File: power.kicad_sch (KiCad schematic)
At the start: 28 parts, among them J2 USB_C_Receptacle_USB2.0, U4 XC6220B331MR, U5 TLV70237_SOT23-5, U6 SRV05-4

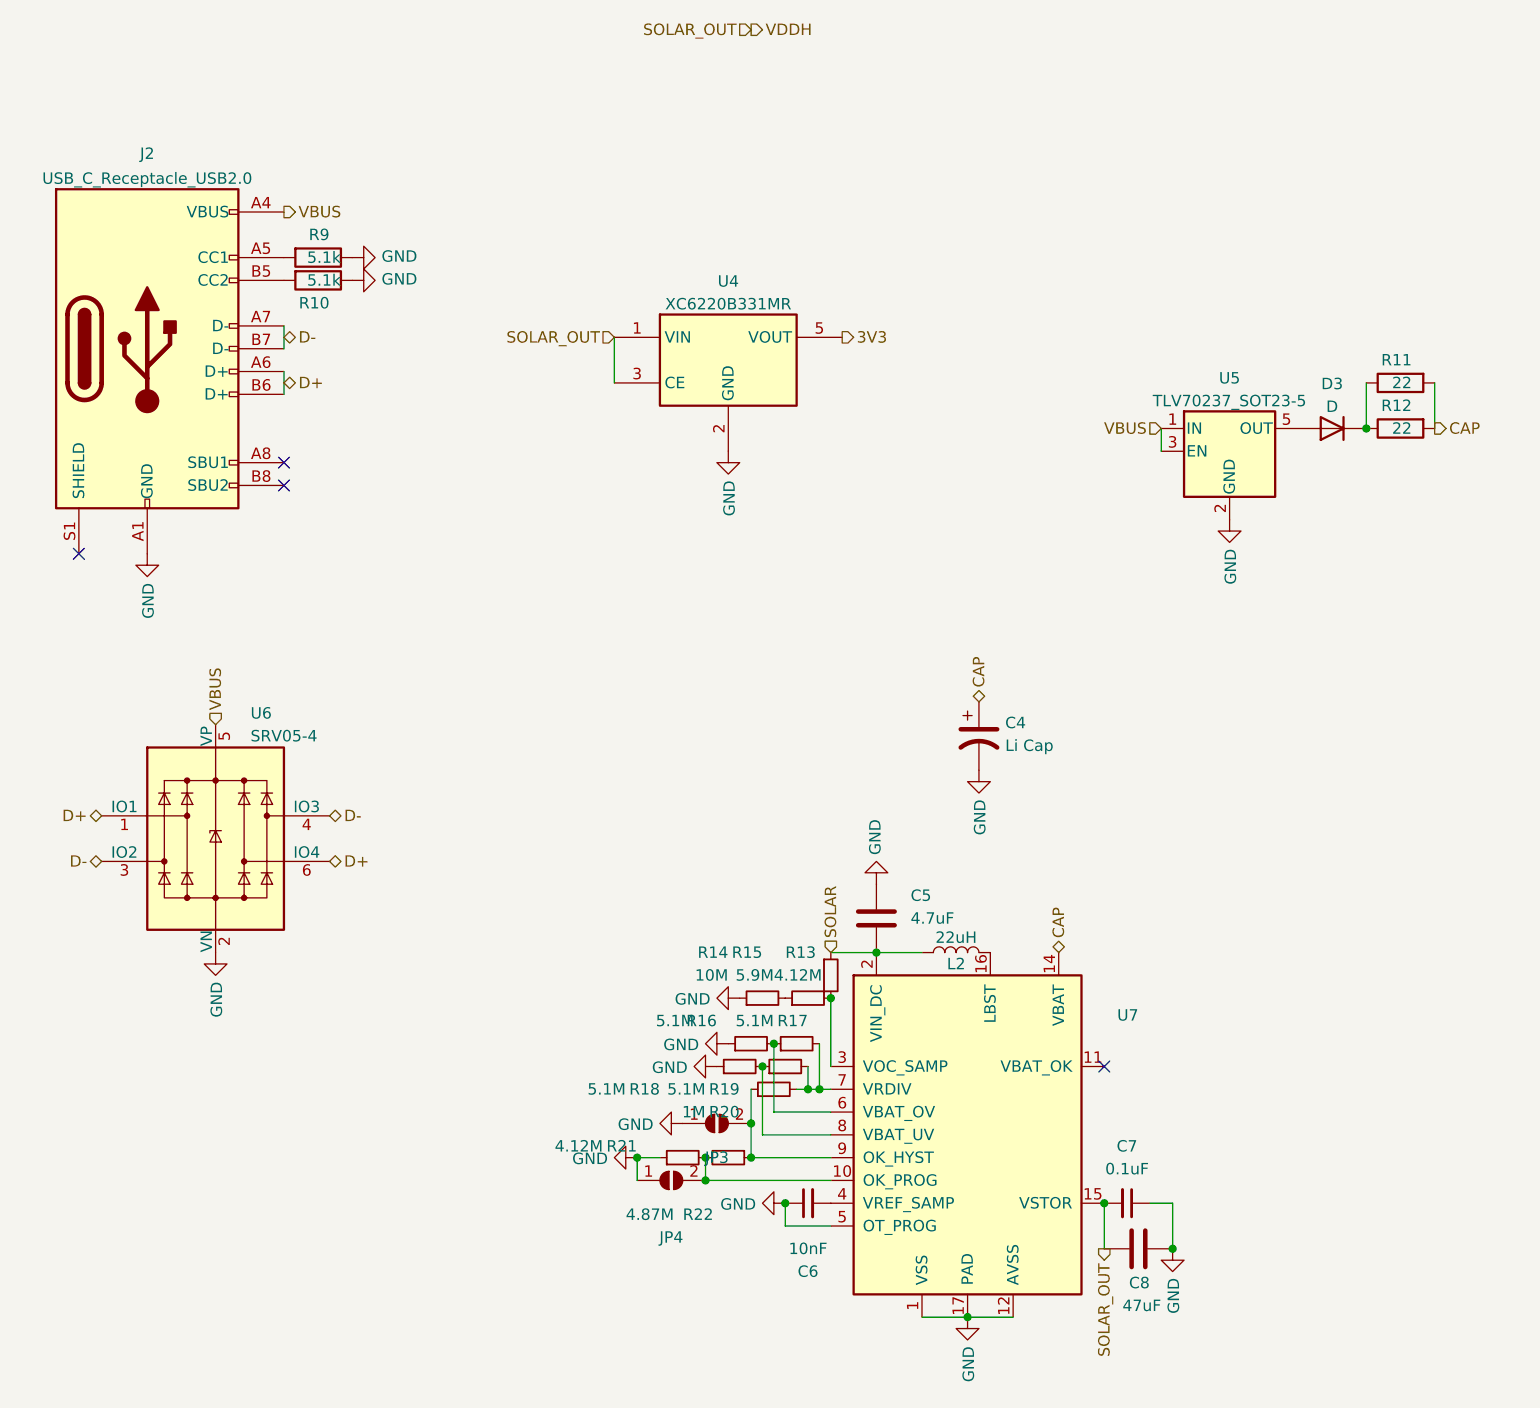
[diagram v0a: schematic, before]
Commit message: no screen
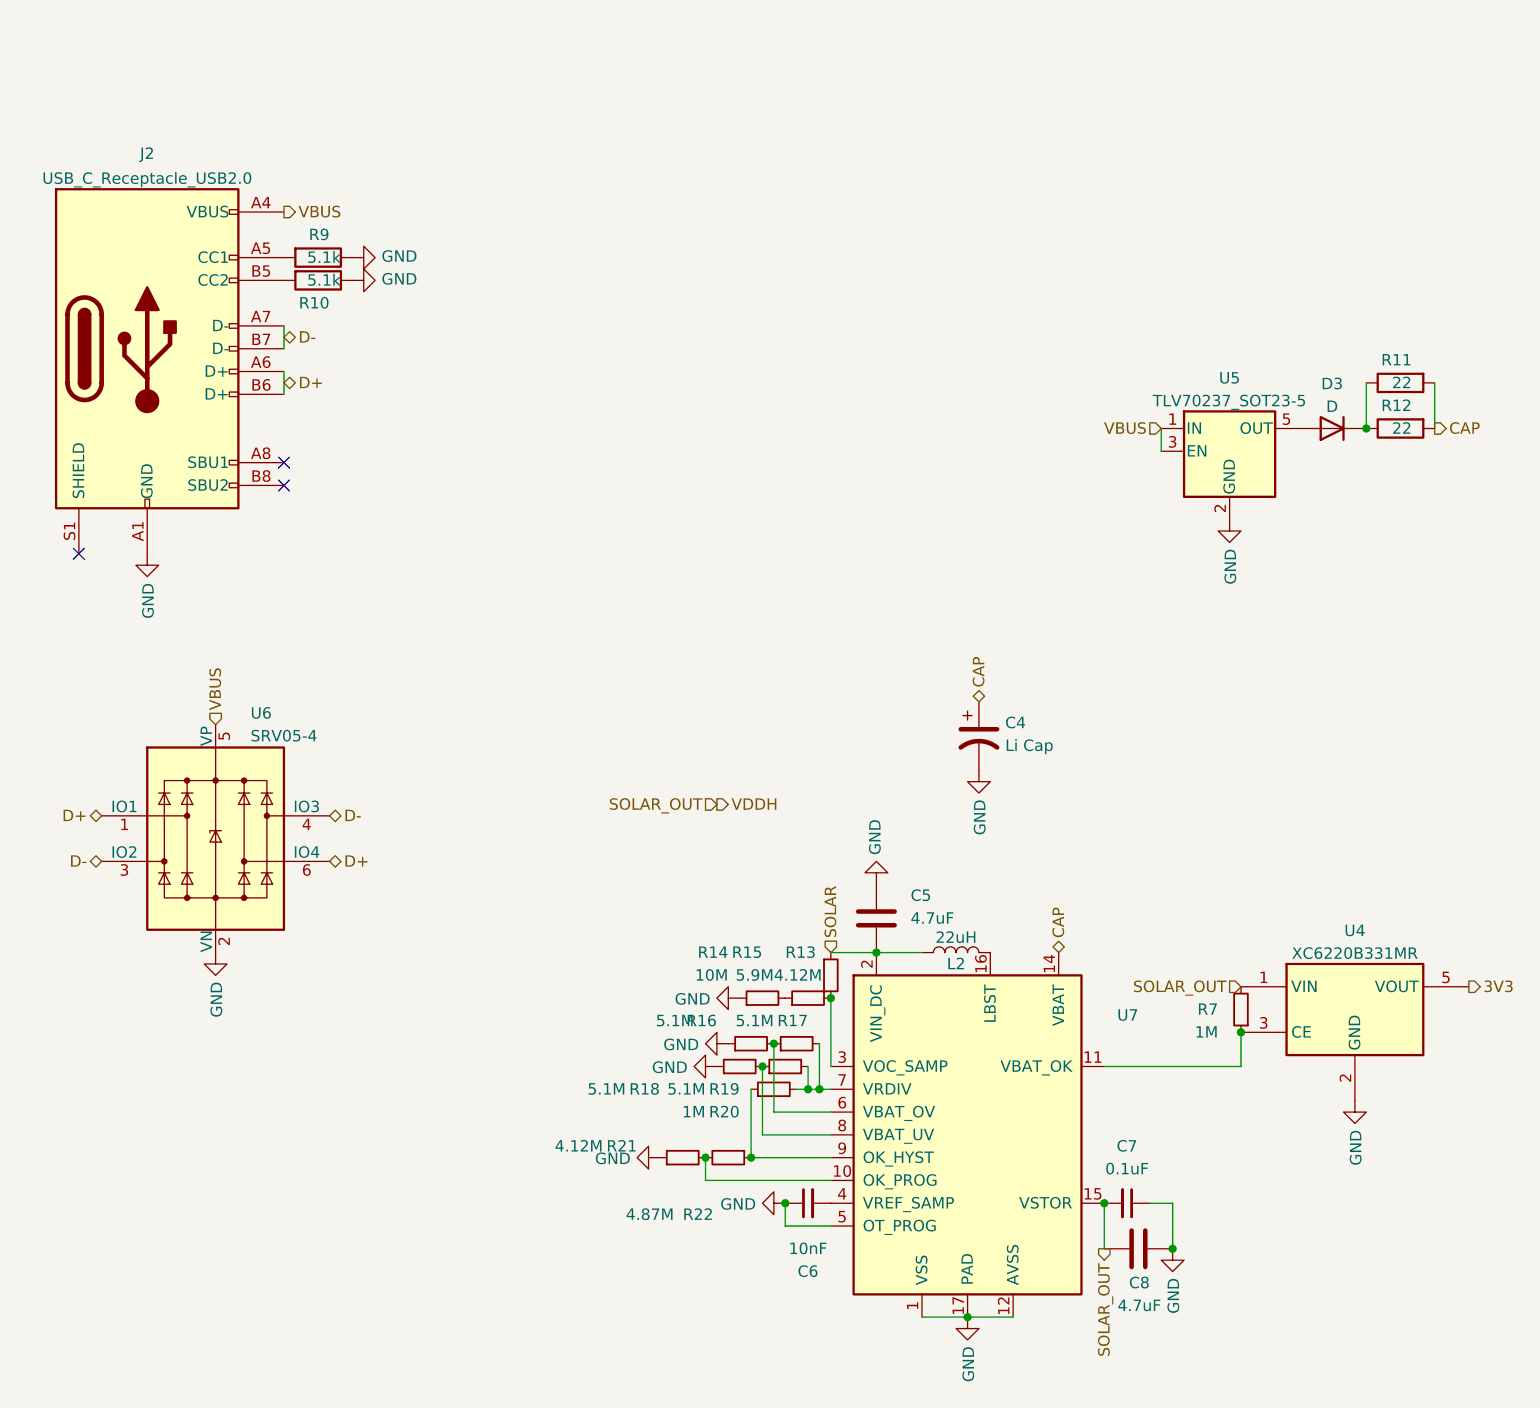
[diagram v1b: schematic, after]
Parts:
- removed JP3: ~, Jumper:SolderJumper-2_P1.3mm_Open_RoundedPad1.0x1.5mm, symbol Jumper:SolderJumper_2_Open
- removed JP4: SolderJumper_2_Open, Jumper:SolderJumper-2_P1.3mm_Open_RoundedPad1.0x1.5mm, symbol Jumper:SolderJumper_2_Open
- added R7: 1M, Resistor_SMD:R_0603_1608Metric, symbol Device:R_Small
- C4: footprint Capacitor_THT:CP_Radial_D13.0mm_P5.00mm -> Capacitor_THT:CP_Radial_D16.0mm_P7.50mm
- C8: value 47uF -> 4.7uF
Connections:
- net SOLAR_OUT: now also R7.2; no longer U4.3 (CE)
- net at U7.11 (VBAT_OK): now also U4.3 (CE), R7.1
- no-connect marks 4 -> 3
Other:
- moved on the sheet: U4
